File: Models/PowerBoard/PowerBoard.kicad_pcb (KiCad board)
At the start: 2 copper layers, 85.8 x 48.2 mm, 53 parts, among them J1 Conn_Coaxial, J10 Conn_01x03_Pin, J11 Conn_01x13_Socket, J12 Banana Socket, Green, J13 Banana Socket, Black, J14 Banana Socket, Blue, J2 Conn_Coaxial, J3 Conn_Coaxial, J4 Conn_Coaxial, J5 Conn_01x03_Pin, J6 Conn_01x03_Pin, J7 Conn_01x03_Pin, J8 Conn_01x03_Pin, J9 Conn_01x03_Pin, U1 LM7815, 15V, 5%, U2 LM7805, 5V, 5%, U3 LM7915, -15V, 5%, U4 TLV76133, 3.3V, 1%, U5 LM7805, 5V, 5%, U6 LM7905, -5V, 5%

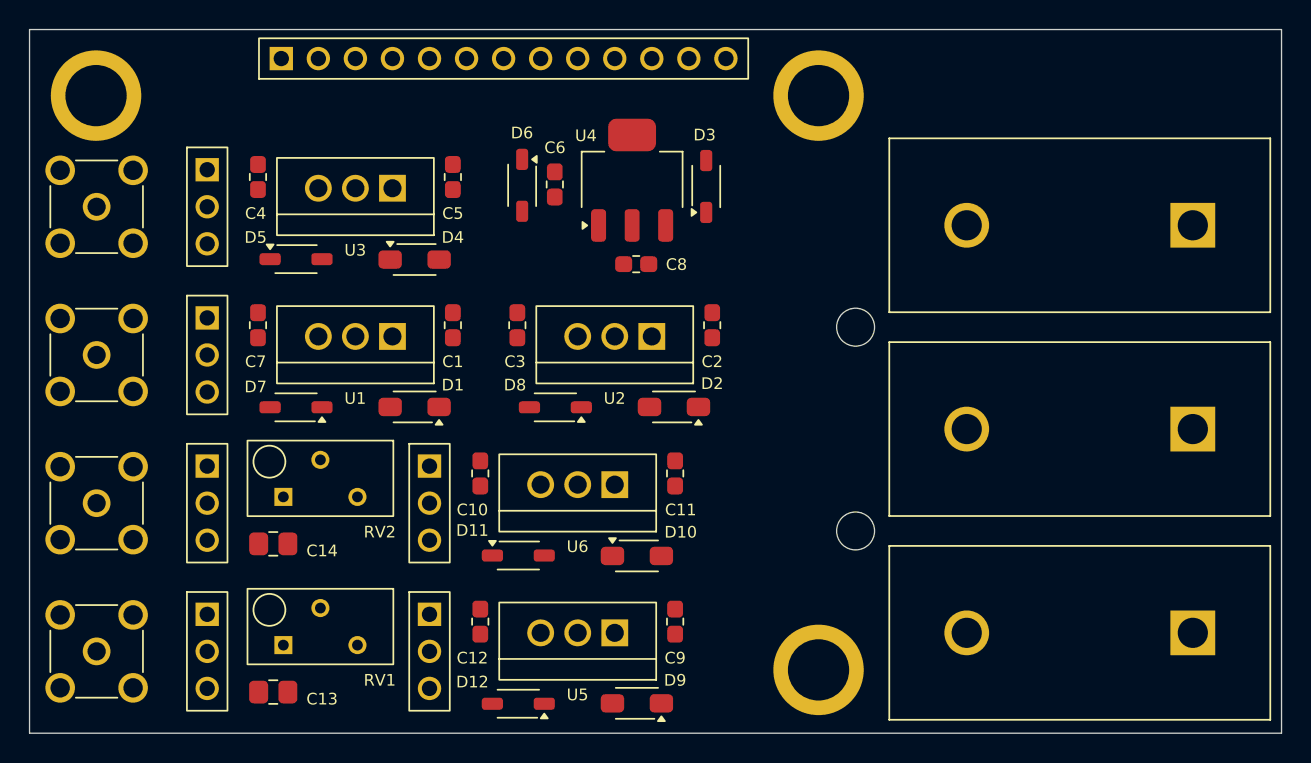
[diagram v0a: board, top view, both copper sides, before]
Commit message: Finished layout of power board
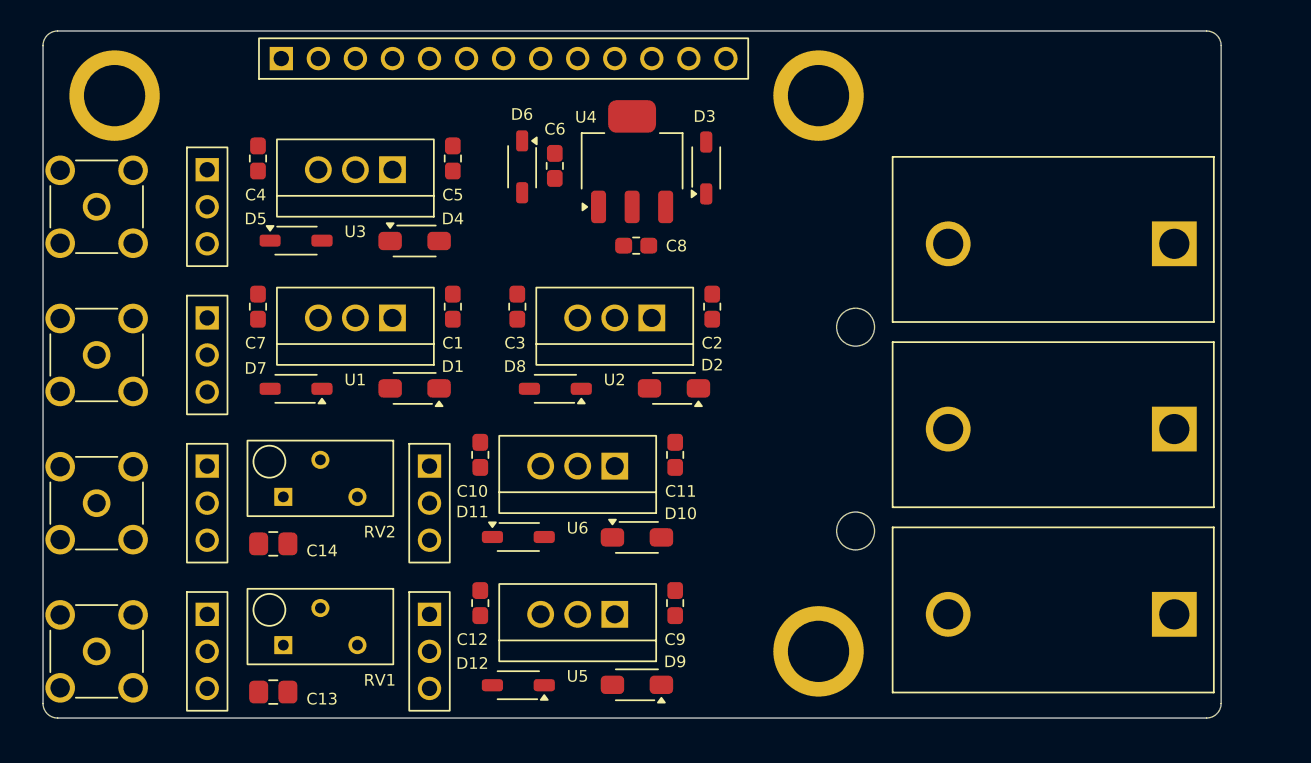
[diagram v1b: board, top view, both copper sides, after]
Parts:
- J12: value Banana Socket, Green -> Banana Socket, Red
- J14: value Banana Socket, Blue -> Banana Socket, Yellow
- moved J12 1.80 mm to (196.6, 71.2)
- moved J14 1.80 mm to (196.6, 45.8)
- moved D10 1.27 mm to (167.5, 65.9)
- moved H1 1.27 mm to (131.7, 35.6)
- moved H4 1.27 mm to (179.9, 73.7)
- moved C1 1.27 mm to (154.8, 50.1)
- moved C2 1.27 mm to (172.6, 50.1)
- moved C3 1.27 mm to (159.3, 50.1)
- moved C7 1.27 mm to (141.5, 50.1)
- moved C8 1.27 mm to (167.4, 45.9)
- moved D1 1.27 mm to (152.2, 55.7)
- moved D2 1.27 mm to (170.0, 55.7)
- moved D5 1.27 mm to (144.1, 45.6)
- moved U3 1.27 mm to (148.2, 40.7)
- moved U6 1.27 mm to (163.4, 61.0)
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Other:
- board size 85.8 x 48.2 mm -> 80.8 x 47.1 mm
